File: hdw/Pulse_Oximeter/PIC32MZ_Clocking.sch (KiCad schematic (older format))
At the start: 16 parts

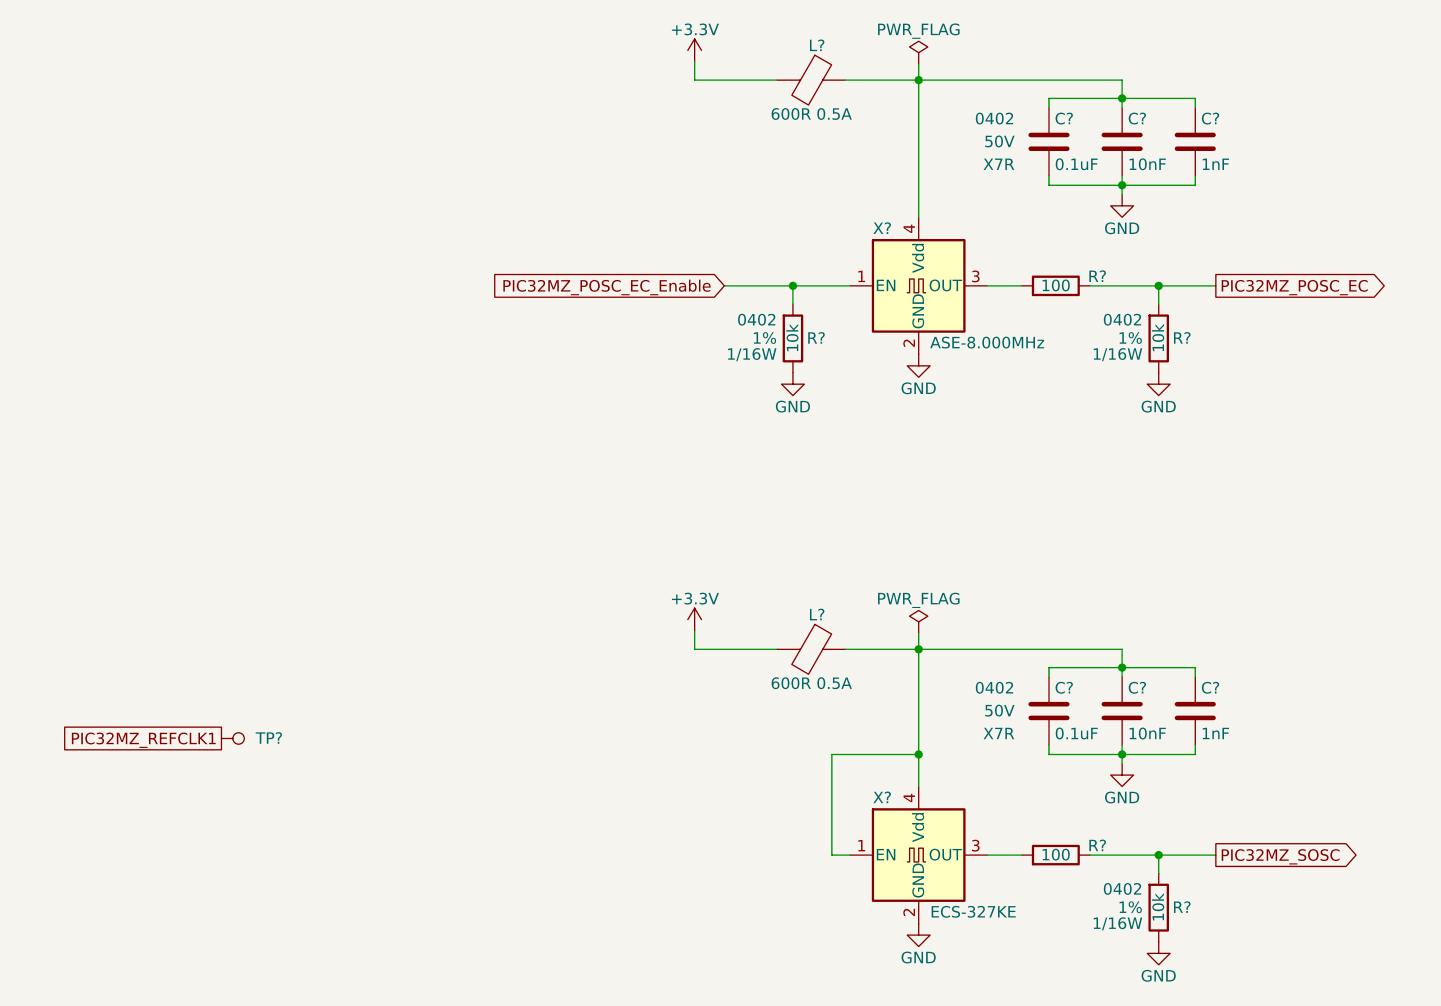
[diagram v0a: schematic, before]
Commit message: More sch work
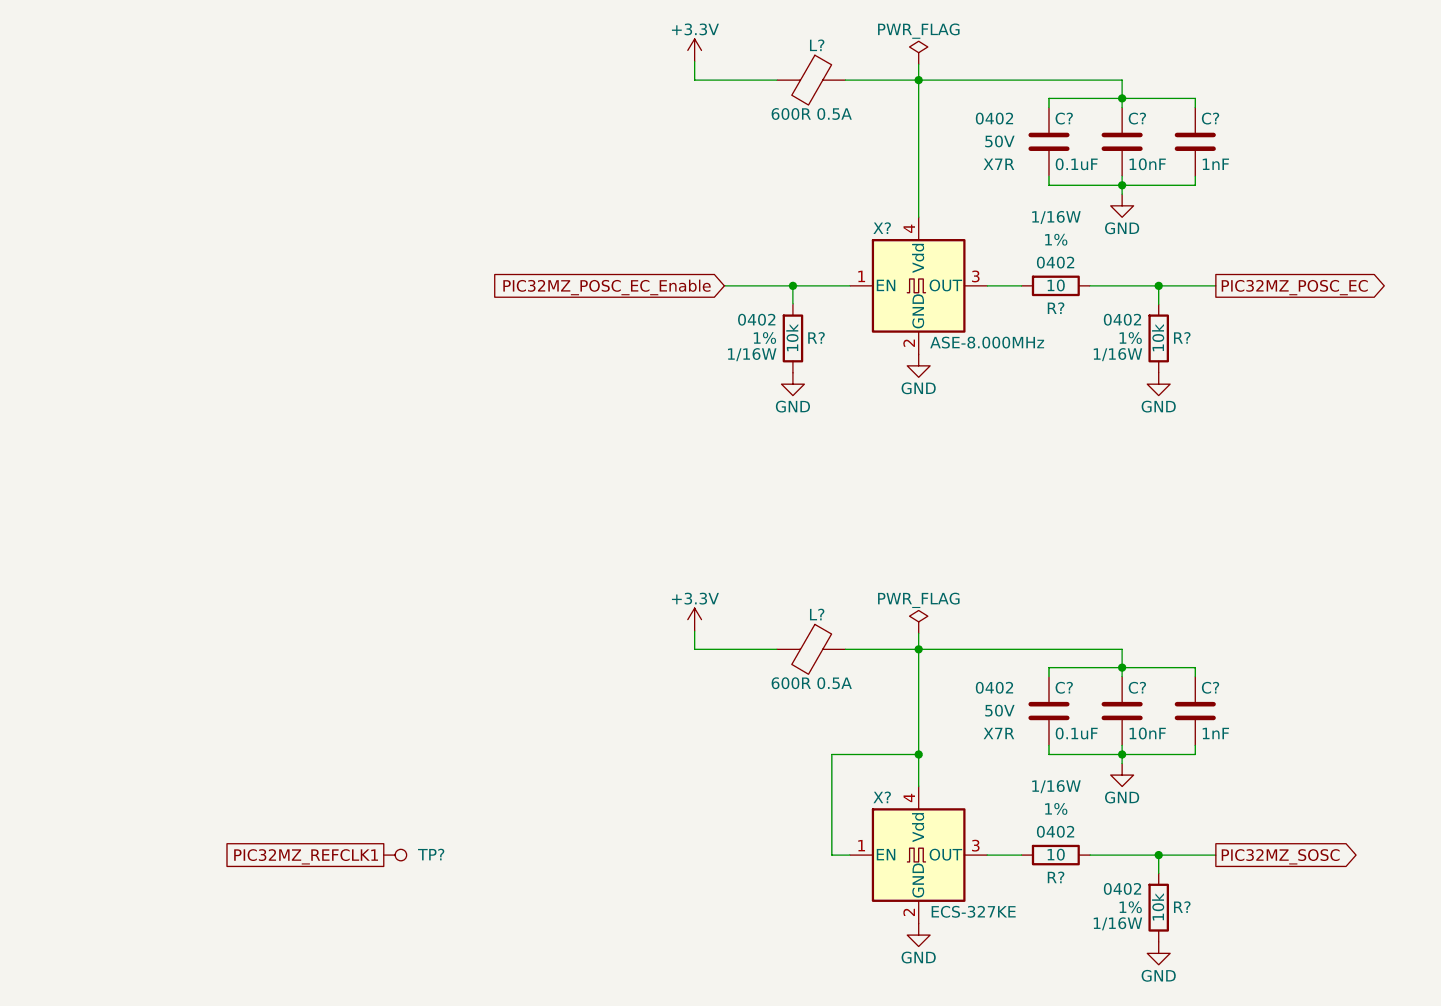
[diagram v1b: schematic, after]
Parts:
- removed R? (x2): 100, Resistors_SMD:R_0402, symbol Custom_Library:R_Custom
- added R? (x2): 10, Resistors_SMD:R_0402, symbol Custom_Library:R_Custom
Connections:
- net PIC32MZ_POSC_EC: now also R?.2
- net PIC32MZ_SOSC: now also R?.2
- net at X?.3 (OUT): now also R?.1 (x2)
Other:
- moved on the sheet: TP?
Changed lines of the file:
@@
 	6560 2700 6560 2780
 Connection ~ 6560 2700
-$Comp
-L Custom_Library:R_Custom R?
-U 1 1 5E024C29
-P 6110 2700
-AR Path="/5BAAE2B6/5E024C29" Ref="R?"  Part="1"
-AR Path="/5BB6CF6D/5E024C29" Ref="R?"  Part="1"
-AR Path="/5BBE424C/5E024C29" Ref="R?"  Part="1"
-AR Path="/5BAAE1DC/5E024C29" Ref="R?"  Part="1"
-AR Path="/5CAD2DA3/5E024C29" Ref="R?"  Part="1"
-AR Path="/5E01BCC3/5E024C29" Ref="R?"  Part="1"
-AR Path="/5E697952/5E024C29" Ref="R?"  Part="1"
-AR Path="/5EAE2F15/5E024C29" Ref="R?"  Part="1"
-F 0 "R?" V 6070 2560 50  0000 R CNN
-F 1 "100" V 6110 2700 50  0000 C CNN
-F 2 "Resistors_SMD:R_0402" H 6110 2700 50  0001 C CNN
-F 3 "" H 6110 2700 50  0001 C CNN
-F 4 "0402" V 6210 2700 50  0001 C CNN "display_footprint"
-F 5 "1%" V 6310 2700 50  0001 C CNN "Tolerance"
-F 6 "1/16W" V 6410 2700 50  0001 C CNN "Wattage"
-F 7 "541-100LCT-ND" H 6410 3100 60  0001 C CNN "Digi-Key PN"
-	1    6110 2700
-	0    -1   1    0
-$EndComp
 Wire Wire Line
 	5960 2700 5810 2700
@@
 	6560 5190 6560 5270
 Connection ~ 6560 5190
-$Comp
-L Custom_Library:R_Custom R?
-U 1 1 5E0562C1
-P 6110 5190
-AR Path="/5BAAE2B6/5E0562C1" Ref="R?"  Part="1"
-AR Path="/5BB6CF6D/5E0562C1" Ref="R?"  Part="1"
-AR Path="/5BBE424C/5E0562C1" Ref="R?"  Part="1"
-AR Path="/5BAAE1DC/5E0562C1" Ref="R?"  Part="1"
-AR Path="/5CAD2DA3/5E0562C1" Ref="R?"  Part="1"
-AR Path="/5E01BCC3/5E0562C1" Ref="R?"  Part="1"
-AR Path="/5E697952/5E0562C1" Ref="R?"  Part="1"
-AR Path="/5EAE2F15/5E0562C1" Ref="R?"  Part="1"
-F 0 "R?" V 6070 5050 50  0000 R CNN
-F 1 "100" V 6110 5190 50  0000 C CNN
-F 2 "Resistors_SMD:R_0402" H 6110 5190 50  0001 C CNN
-F 3 "" H 6110 5190 50  0001 C CNN
-F 4 "0402" V 6210 5190 50  0001 C CNN "display_footprint"
-F 5 "1%" V 6310 5190 50  0001 C CNN "Tolerance"
-F 6 "1/16W" V 6410 5190 50  0001 C CNN "Wattage"
-F 7 "541-100LCT-ND" H 6410 5590 60  0001 C CNN "Digi-Key PN"
-	1    6110 5190
-	0    -1   1    0
-$EndComp
 Wire Wire Line
 	5960 5190 5810 5190
@@
 L Custom_Library:TP TP?
 U 1 1 5EBAE156
-P 2460 4680
+P 3170 5190
 AR Path="/5C1D5CD8/5EBAE156" Ref="TP?"  Part="1"
 AR Path="/5C1D5C9E/5EBAE156" Ref="TP?"  Part="1"
@@
 AR Path="/5EAE2D66/5EBAE156" Ref="TP?"  Part="1"
 AR Path="/5EAE2F15/5EBAE156" Ref="TP?"  Part="1"
-F 0 "TP?" V 2460 4830 50  0000 L CNN
-F 1 "TP" H 2460 4830 50  0001 C CNN
-F 2 "Custom Footprints Library:Test_Point" H 2460 4680 60  0001 C CNN
-F 3 "" H 2460 4680 60  0000 C CNN
-	1    2460 4680
+F 0 "TP?" V 3170 5340 50  0000 L CNN
+F 1 "TP" H 3170 5340 50  0001 C CNN
+F 2 "Custom Footprints Library:Test_Point" H 3170 5190 60  0001 C CNN
+F 3 "" H 3170 5190 60  0000 C CNN
+	1    3170 5190
 	0    1    1    0
 $EndComp
-Text GLabel 2460 4680 0    50   UnSpc ~ 0
+Text GLabel 3170 5190 0    50   UnSpc ~ 0
 PIC32MZ_REFCLK1
+$Comp
+L Custom_Library:R_Custom R?
+U 1 1 5EB9D3C3
+P 6110 5190
+AR Path="/5EAE2EF2/5EB9D3C3" Ref="R?"  Part="1"
+AR Path="/5EAE2F15/5EB9D3C3" Ref="R?"  Part="1"
+F 0 "R?" V 6010 5190 50  0000 C CNN
+F 1 "10" V 6110 5190 50  0000 C CNN
+F 2 "Resistors_SMD:R_0402" H 6110 5190 50  0001 C CNN
+F 3 "" H 6110 5190 50  0001 C CNN
+F 4 "0402" V 6210 5190 50  0000 C CNN "display_footprint"
+F 5 "1%" V 6310 5190 50  0000 C CNN "Tolerance"
+F 6 "1/16W" V 6410 5190 50  0000 C CNN "Wattage"
+F 7 "541-3964-1-ND" H 6410 5590 60  0001 C CNN "Digi-Key PN"
+	1    6110 5190
+	0    -1   -1   0
+$EndComp
+$Comp
+L Custom_Library:R_Custom R?
+U 1 1 5EB9DF29
+P 6110 2700
+AR Path="/5EAE2EF2/5EB9DF29" Ref="R?"  Part="1"
+AR Path="/5EAE2F15/5EB9DF29" Ref="R?"  Part="1"
+F 0 "R?" V 6010 2700 50  0000 C CNN
+F 1 "10" V 6110 2700 50  0000 C CNN
+F 2 "Resistors_SMD:R_0402" H 6110 2700 50  0001 C CNN
+F 3 "" H 6110 2700 50  0001 C CNN
+F 4 "0402" V 6210 2700 50  0000 C CNN "display_footprint"
+F 5 "1%" V 6310 2700 50  0000 C CNN "Tolerance"
+F 6 "1/16W" V 6410 2700 50  0000 C CNN "Wattage"
+F 7 "541-3964-1-ND" H 6410 3100 60  0001 C CNN "Digi-Key PN"
+	1    6110 2700
+	0    -1   -1   0
+$EndComp
 $EndSCHEMATC
